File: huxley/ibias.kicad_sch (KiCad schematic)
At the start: 24 parts, among them J21 61300211121, J25 61300211121, J26 61300211121, J27 61300211121, J28 61300211121, J29 61300211121, J30 61300211121, J31 61300211121, U2 LM134H, U4 TMUX1112PWR, U5 TMUX1112PWR

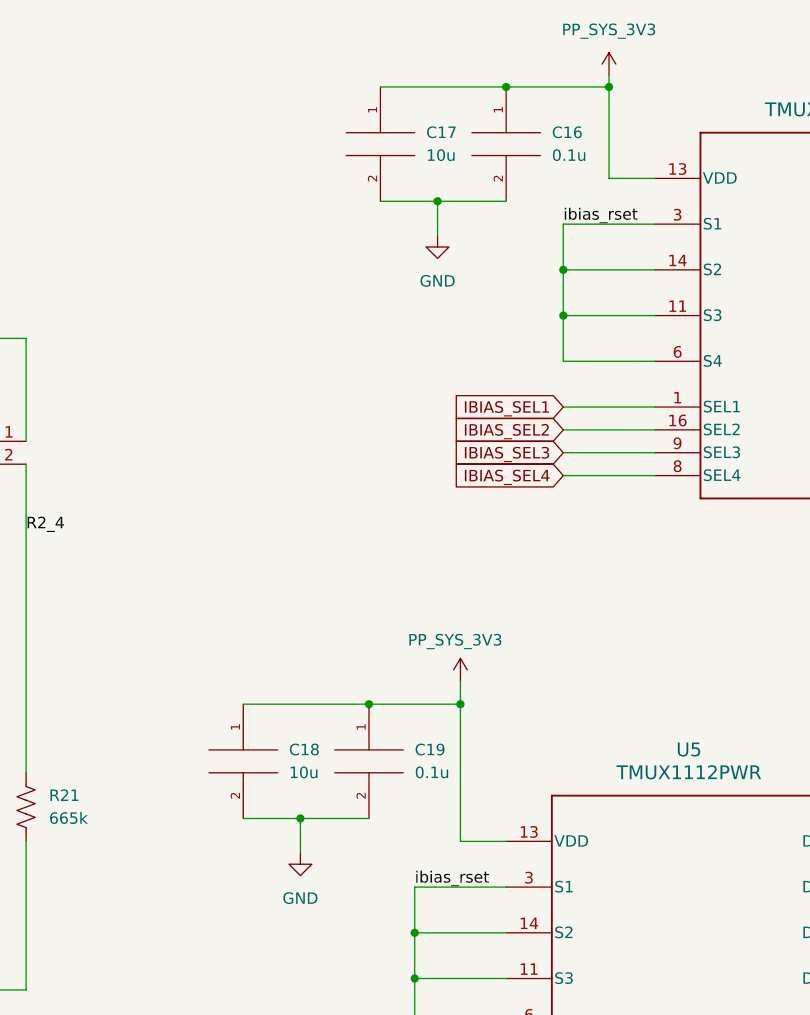
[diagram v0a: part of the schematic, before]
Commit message: layout_1010
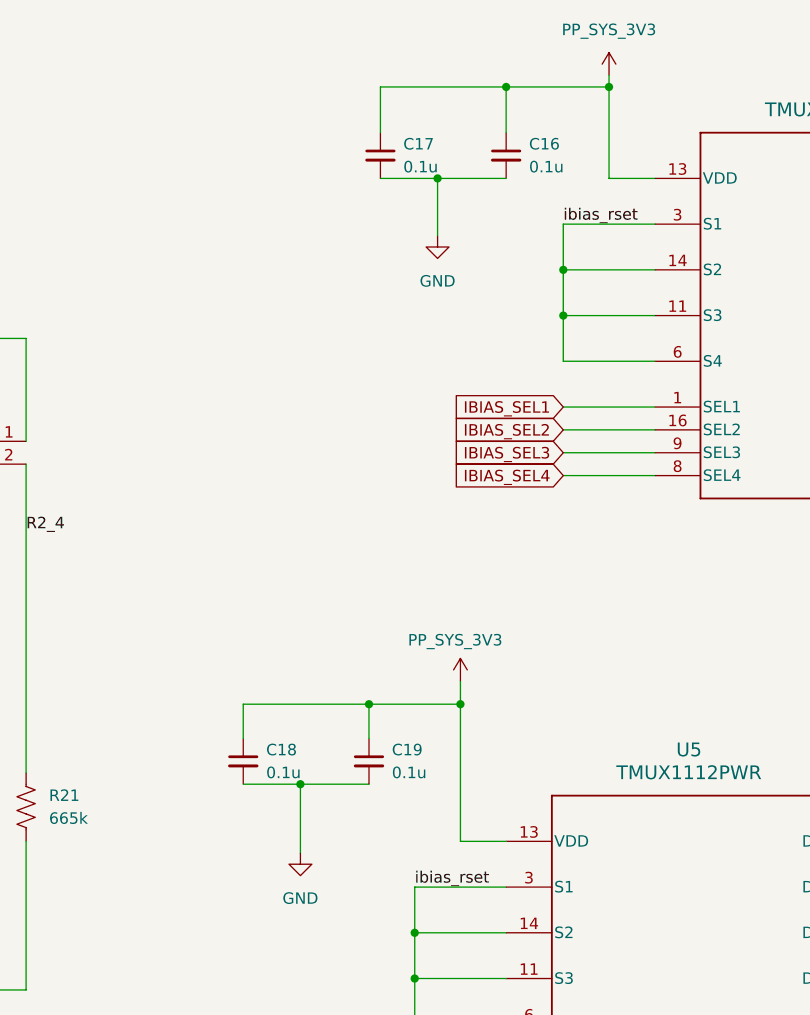
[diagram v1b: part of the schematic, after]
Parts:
- C16, C19: symbol pspice:C -> Device:C_Small
- C17, C18: value 10u -> 0.1u; symbol pspice:C -> Device:C_Small
- U2: footprint 0_726_footprints:lm134 -> Package_TO_SOT_THT:TO-46-3
